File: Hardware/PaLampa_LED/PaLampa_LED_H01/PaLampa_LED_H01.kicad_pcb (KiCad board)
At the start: 2 copper layers, 59 x 73 mm, 77 parts, among them J1 Conn_02x04_Odd_Even, J2 Conn_01x03, U1 DS18B20

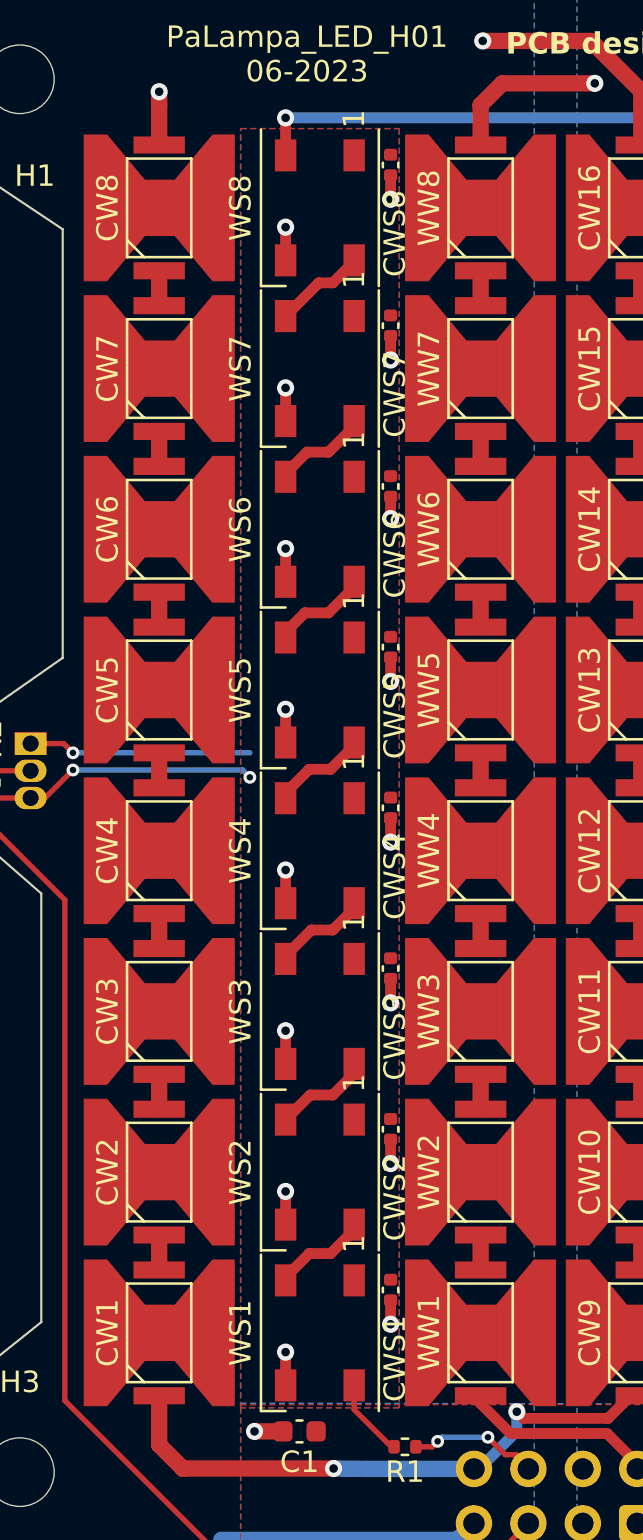
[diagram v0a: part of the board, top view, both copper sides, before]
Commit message: H01 update
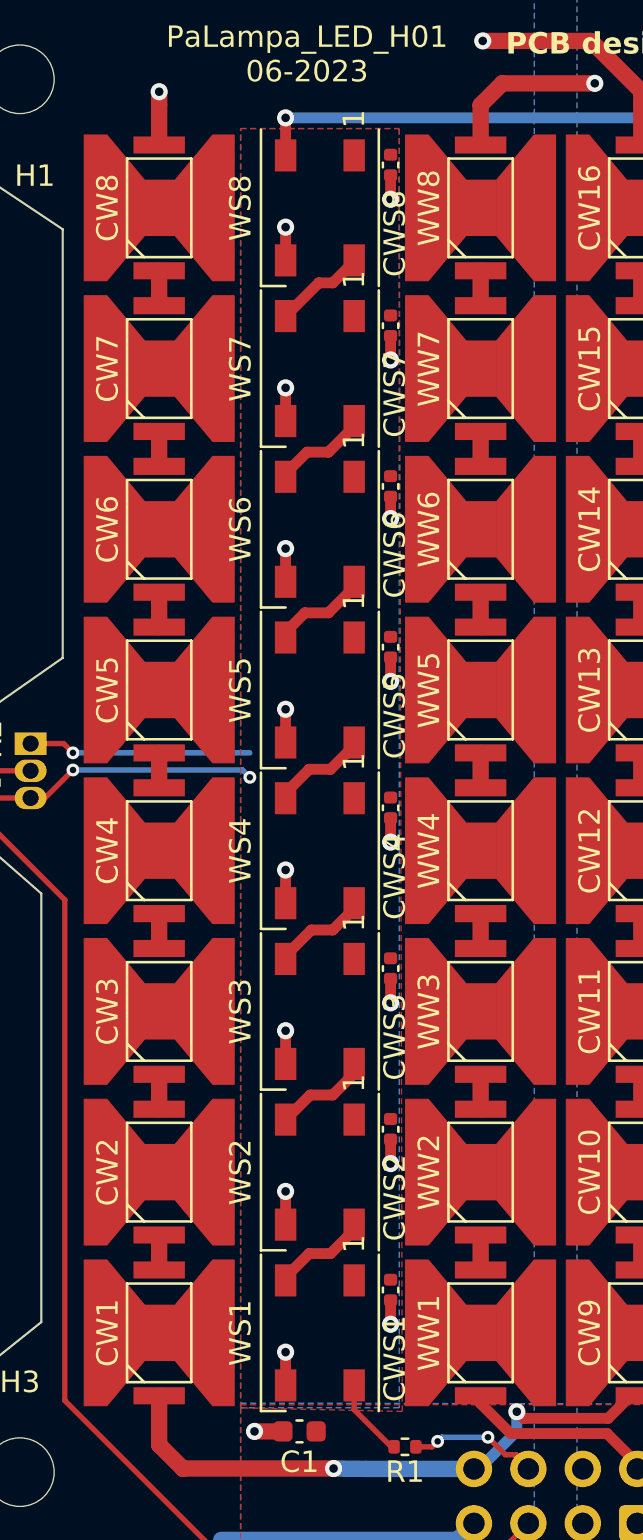
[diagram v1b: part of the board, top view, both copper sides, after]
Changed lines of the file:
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@@
     (polygon
       (pts
-        (xy 21.7 66)
+        (xy 21.844 66.167)
         (xy 14.3 66)
         (xy 14.3 6.3)
